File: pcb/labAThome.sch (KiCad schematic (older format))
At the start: 107 parts, among them J1 I2C, J11 24.5.GND.3, J12 NEOPIXEL, J13 Power Input 1, J14 Conn_Coaxial, J15 WS2812_OUT, J2 SRVx, J3 5V, J4 EXT, J5 VPS, J6 FAN2, J7 1wire, J8 1wire, J9 FAN1, K1 G5V-2, K2 G5V-2, K3 G5V-2, M3 SN65HVD230_MODULE, Q1 BC847, Q2 IRLZ44N, Q3 IRLML6344, Q4 BC847, Q5 IRF530, Q6 IRLML5203, SW1 RED, SW2 GREEN, SW4 BLUE, SW5 WHITE, SW7 ROTENC, U1 SR602, U10 MAX3485_MODULE, U11 AM312, U12 24V->4V, U13 LM358, U14 MS4525DO, U15 CCS811_MODULE, U16 24V->5V, U17 DS18B20, U2 TPS5430DDA, U3 Power Input 2, U4 ESP32_DEVKITC_COMPATIBLE, U6 GY-302, U7 Display, U8 MIC, U9 RFM95W-868S2, X1 FAN_6024, m1 Attribution

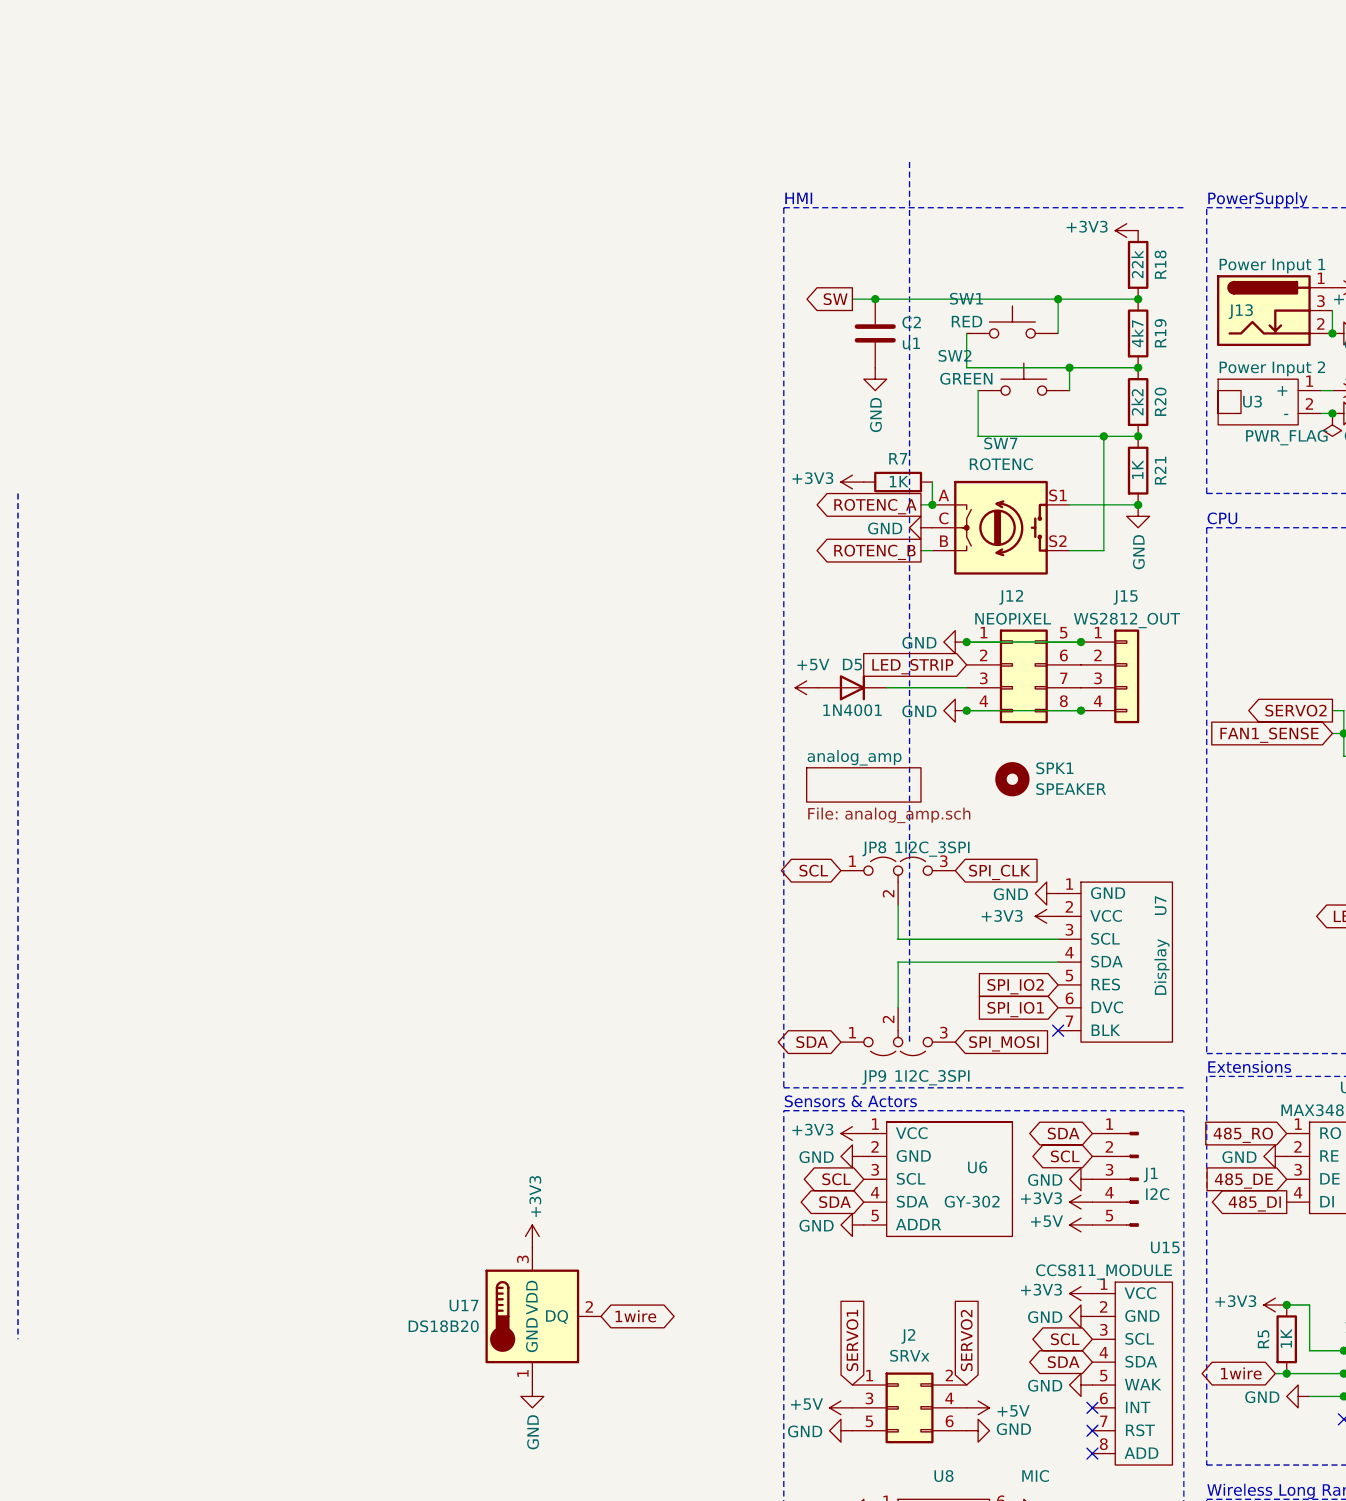
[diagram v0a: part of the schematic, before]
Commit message: Minor PCB update
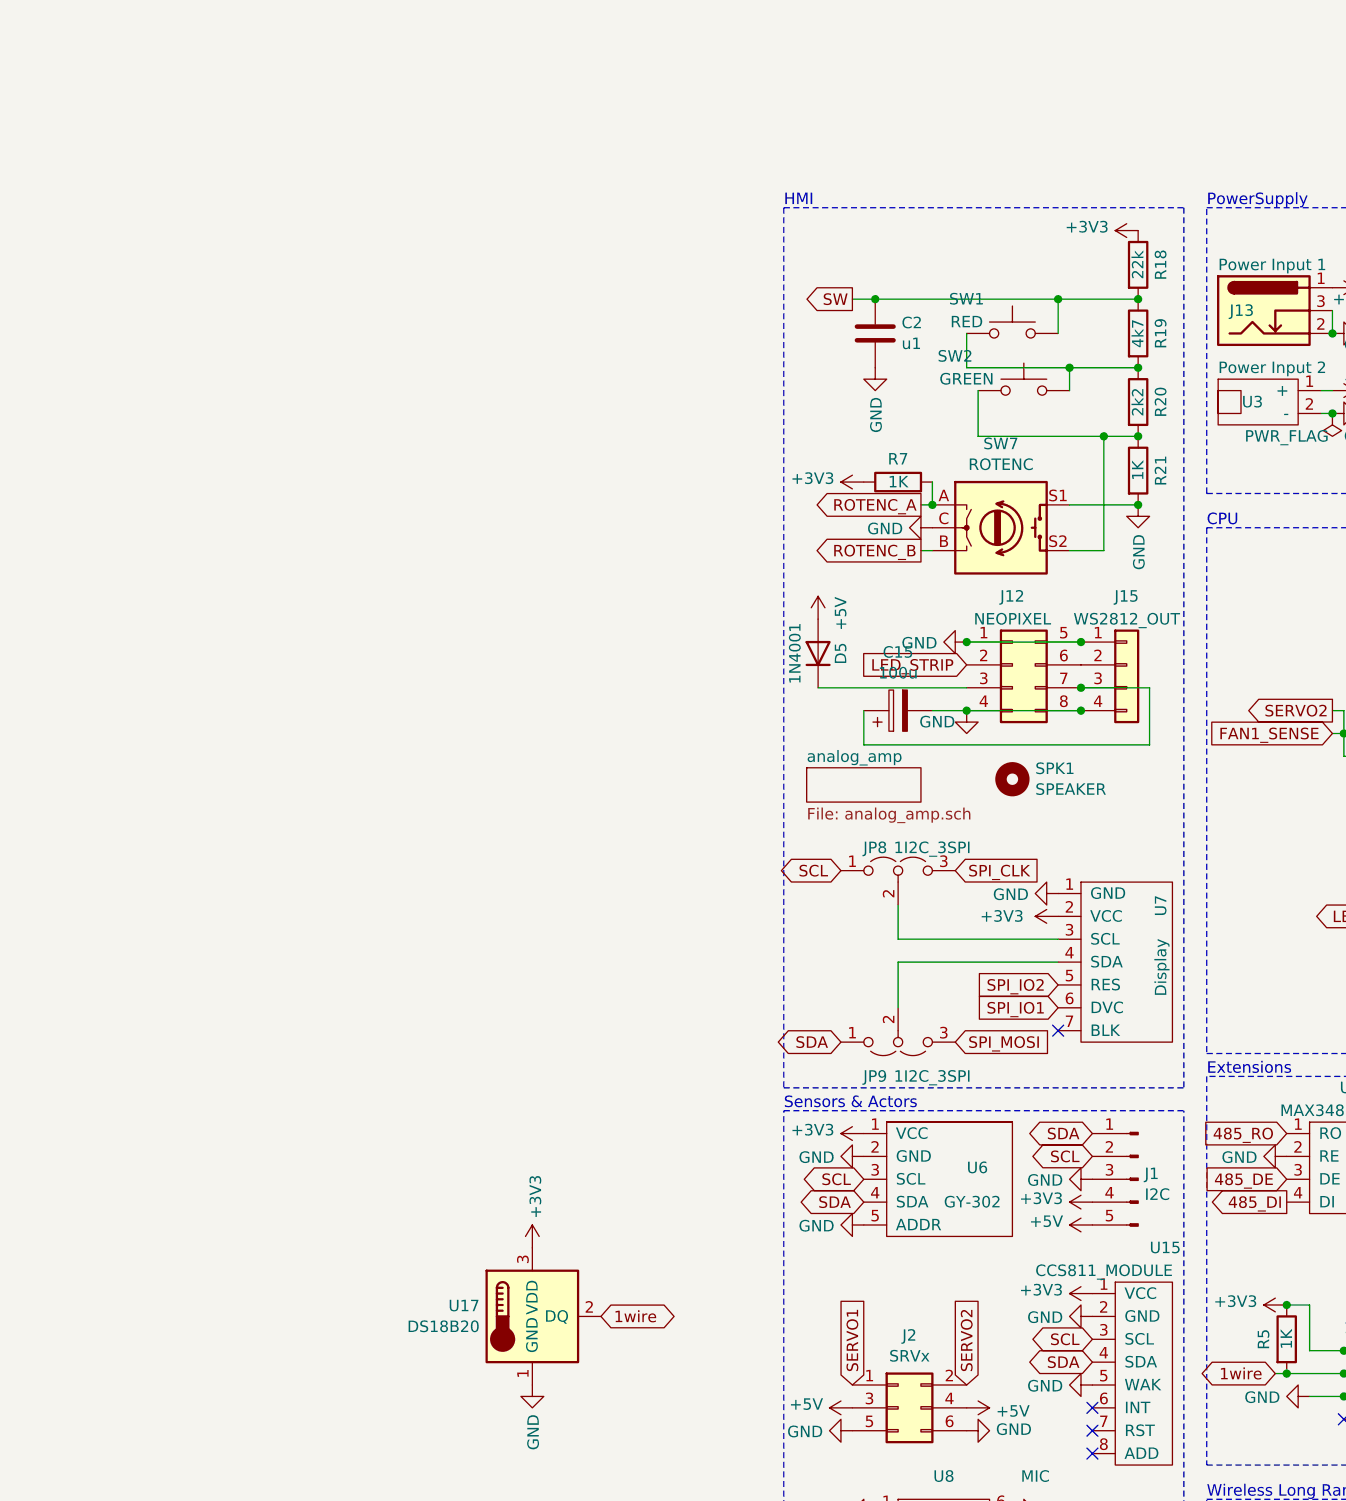
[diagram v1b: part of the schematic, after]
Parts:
- added C15: 100u, liebler_PASSIVES:CP_Elec_6.3x7.7_handsolder, symbol Device:CP
- J12: footprint smopla:NEOPIXEL_STICK_alternativ -> liebler_MODULES:NEOPIXEL_STICK
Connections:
- net GND: now also C15.2
- net at J12.7 (Pin_7), J15.3 (Pin_3): now also C15.1
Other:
- moved on the sheet: D5
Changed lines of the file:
@@
 	1    0    0    -1
 $EndComp
-Wire Notes Line
-	-2800 1850 -2800 5550
 $Comp
 L power:GND #PWR0109
@@
 L power:+5V #PWR051
 U 1 1 5EFC1FD4
-P 700 2700
-F 0 "#PWR051" H 700 2550 50  0001 C CNN
-F 1 "+5V" V 800 2650 50  0000 L CNN
-F 2 "" H 700 2700 50  0001 C CNN
-F 3 "" H 700 2700 50  0001 C CNN
-	1    700  2700
-	0    -1   -1   0
+P 700 2400
+F 0 "#PWR051" H 700 2250 50  0001 C CNN
+F 1 "+5V" V 800 2350 50  0000 L CNN
+F 2 "" H 700 2400 50  0001 C CNN
+F 3 "" H 700 2400 50  0001 C CNN
+	1    700  2400
+	1    0    0    -1
 $EndComp
 $Comp
@@
 P 1350 2800
 F 0 "#PWR052" H 1350 2550 50  0001 C CNN
-F 1 "GND" V 1355 2672 50  0000 R CNN
+F 1 "GND" H 1300 2750 50  0000 R CNN
 F 2 "" H 1350 2800 50  0001 C CNN
 F 3 "" H 1350 2800 50  0001 C CNN
 	1    1350 2800
-	0    1    1    0
+	1    0    0    -1
 $EndComp
 $Comp
@@
 L Diode:1N4001 D5
 U 1 1 5EFF290C
-P 850 2700
-F 0 "D5" H 850 2600 50  0000 C CNN
-F 1 "1N4001" H 850 2800 50  0000 C CNN
-F 2 "Diode_SMD:D_SMA_Handsoldering" H 850 2525 50  0001 C CNN
-F 3 "http://www.vishay.com/docs/88503/1n4001.pdf" H 850 2700 50  0001 C CNN
-	1    850  2700
-	-1   0    0    1
+P 700 2550
+F 0 "D5" H 700 2450 50  0000 C CNN
+F 1 "1N4001" H 700 2650 50  0000 C CNN
+F 2 "Diode_SMD:D_SMA_Handsoldering" H 700 2375 50  0001 C CNN
+F 3 "http://www.vishay.com/docs/88503/1n4001.pdf" H 700 2550 50  0001 C CNN
+	1    700  2550
+	0    -1   -1   0
 $EndComp
 $Comp
@@
 SPI_IO2
 NoConn ~ 1750 4200
-Wire Wire Line
-	1350 2700 1000 2700
 Wire Wire Line
 	7900 3100 7900 3200
@@
 F 0 "J12" H 1550 2900 50  0000 C CNN
 F 1 "NEOPIXEL" H 1550 2800 50  0000 C CNN
-F 2 "smopla:NEOPIXEL_STICK_alternativ" H 1550 2600 50  0001 C CNN
+F 2 "liebler_MODULES:NEOPIXEL_STICK" H 1550 2600 50  0001 C CNN
 F 3 "~" H 1550 2600 50  0001 C CNN
 	1    1550 2600
@@
 $EndComp
 Wire Notes Line
-	1100 400  1100 4250
+	2300 600  2300 4450
 Wire Notes Line
 	550  600  550  4450
@@
 F1 "analog_amp.sch" 50
 $EndSheet
+$Comp
+L Device:CP C15
+U 1 1 60C23DBB
+P 1050 2800
+F 0 "C15" V 1305 2800 50  0000 C CNN
+F 1 "100u" V 1214 2800 50  0000 C CNN
+F 2 "liebler_PASSIVES:CP_Elec_6.3x7.7_handsolder" H 1088 2650 50  0001 C CNN
+F 3 "~" H 1050 2800 50  0001 C CNN
+	1    1050 2800
+	0    -1   -1   0
+$EndComp
+Wire Wire Line
+	1350 2800 1200 2800
+Wire Wire Line
+	700  2700 1350 2700
+Wire Wire Line
+	1850 2700 2150 2700
+Wire Wire Line
+	2150 2700 2150 2950
+Wire Wire Line
+	2150 2950 900  2950
+Wire Wire Line
+	900  2950 900  2800
+Connection ~ 1850 2700
 $EndSCHEMATC

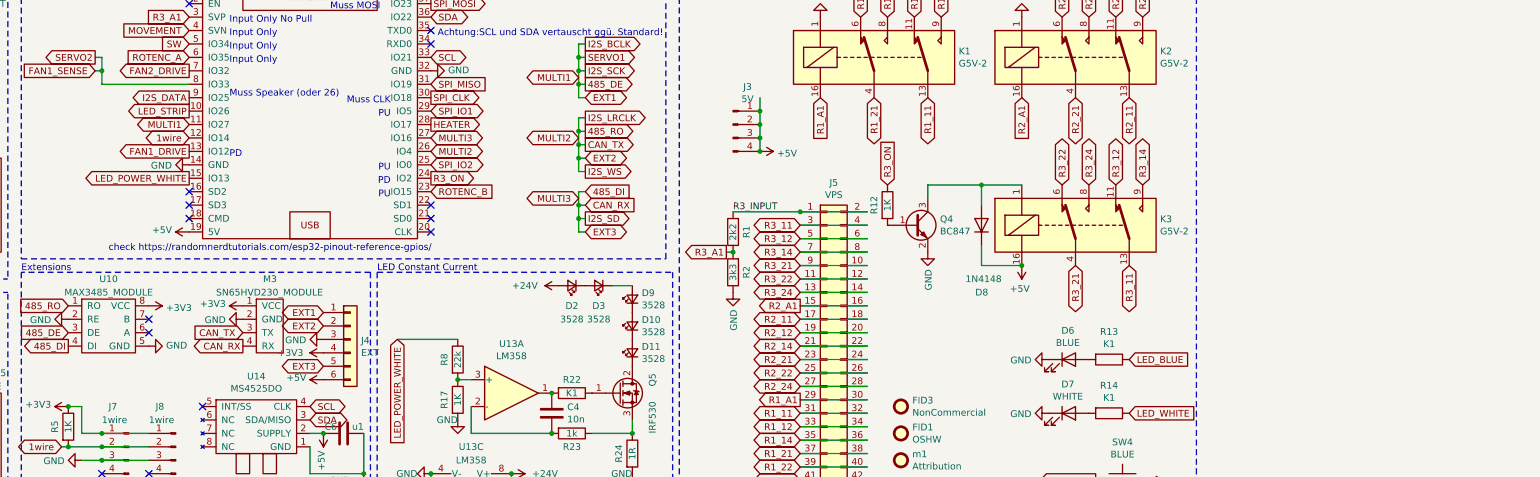
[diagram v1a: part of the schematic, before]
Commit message: labathome V6 as ordered at JLCPCB
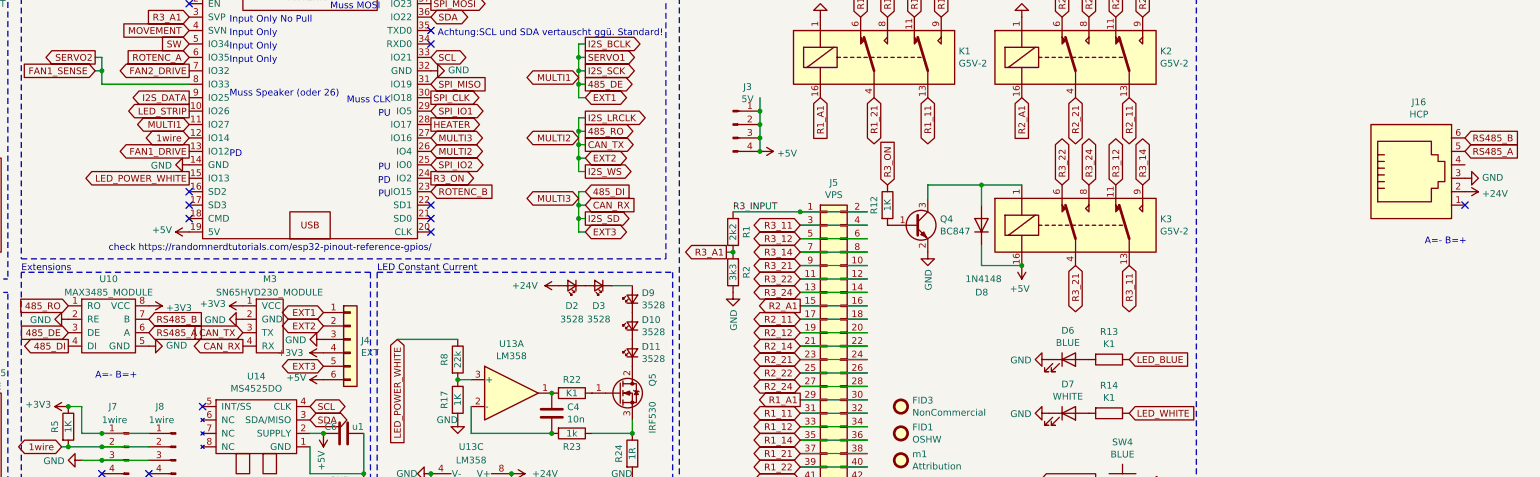
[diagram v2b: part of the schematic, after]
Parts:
- added J16: HCP, liebler_CONN:WR_MJ_Modular_Jack_Vertical_Plastic_6P6C, symbol Connector:6P6C
- SW1, SW2, SW4, SW5: footprint Button_Switch_THT:SW_PUSH-12mm -> liebler_MECH:Button_12mm_ANCHOR_CENTER
- SW7: footprint smopla:RotaryEncoder_Alps_EC11E-Switch_Vertical_H20mm -> liebler_MECH:RotaryEncoder_Alps_EC11E-Switch_Vertical_H20mm
- U1: footprint smopla:SR602 -> liebler_MODULES:PIR_Sensor_SR602
- U4: footprint smopla:ESP32_DEVKITC_COMPATIBLE -> liebler_MODULES:ESP32_DEVKITC_COMPATIBLE
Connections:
- net +24V: now also J16.2
- net GND: now also J16.3
- net RS485_A: now reaches U10.6 (A)
- net RS485_A: now also J16.5
- net RS485_B: now reaches U10.7 (B)
- net RS485_B: now also J16.6
- no-connect marks 33 -> 32
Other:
- note added: "A=- B=+"
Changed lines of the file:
@@
 F 0 "SW1" H 1750 1300 50  0000 C CNN
 F 1 "RED" H 1750 1200 50  0000 C CNN
-F 2 "Button_Switch_THT:SW_PUSH-12mm" H 1550 1350 50  0001 C CNN
+F 2 "liebler_MECH:Button_12mm_ANCHOR_CENTER" H 1550 1350 50  0001 C CNN
 F 3 "~" H 1550 1350 50  0001 C CNN
 	1    1550 1150
@@
 F 0 "SW2" H 1300 1550 50  0000 C CNN
 F 1 "GREEN" H 1350 1450 50  0000 C CNN
-F 2 "Button_Switch_THT:SW_PUSH-12mm" H 1600 1600 50  0001 C CNN
+F 2 "liebler_MECH:Button_12mm_ANCHOR_CENTER" H 1600 1600 50  0001 C CNN
 F 3 "~" H 1600 1600 50  0001 C CNN
 	1    1600 1400
@@
 F 0 "SW5" H 10600 6635 50  0000 C CNN
 F 1 "WHITE" H 10600 6544 50  0000 C CNN
-F 2 "Button_Switch_THT:SW_PUSH-12mm" H 10600 6550 50  0001 C CNN
+F 2 "liebler_MECH:Button_12mm_ANCHOR_CENTER" H 10600 6550 50  0001 C CNN
 F 3 "~" H 10600 6550 50  0001 C CNN
 	1    10600 6350
@@
 F 0 "SW4" H 10600 6235 50  0000 C CNN
 F 1 "BLUE" H 10600 6144 50  0000 C CNN
-F 2 "Button_Switch_THT:SW_PUSH-12mm" H 10600 6150 50  0001 C CNN
+F 2 "liebler_MECH:Button_12mm_ANCHOR_CENTER" H 10600 6150 50  0001 C CNN
 F 3 "~" H 10600 6150 50  0001 C CNN
 	1    10600 5950
@@
 F 0 "U4" H 4550 4325 50  0000 C CNN
 F 1 "ESP32_DEVKITC_COMPATIBLE" H 4550 4234 50  0000 C CNN
-F 2 "smopla:ESP32_DEVKITC_COMPATIBLE" H 4550 3050 50  0001 C CNN
+F 2 "liebler_MODULES:ESP32_DEVKITC_COMPATIBLE" H 4550 3050 50  0001 C CNN
 F 3 "" H 4550 3050 50  0001 C CNN
 	1    4550 3200
@@
 F 0 "U1" H 742 7465 50  0000 C CNN
 F 1 "SR602" H 742 7374 50  0000 C CNN
-F 2 "smopla:SR602" H 800 7100 50  0001 C CNN
+F 2 "liebler_MODULES:PIR_Sensor_SR602" H 800 7100 50  0001 C CNN
 F 3 "" H 800 7100 50  0001 C CNN
 	1    800  7100
@@
 	0    1    1    0
 $EndComp
-NoConn ~ 3350 4850
-NoConn ~ 3350 4750
 $Comp
 L power:GND #PWR0116
@@
 F 0 "SW7" H 1500 2367 50  0000 C CNN
 F 1 "ROTENC" H 1500 2276 50  0000 C CNN
-F 2 "smopla:RotaryEncoder_Alps_EC11E-Switch_Vertical_H20mm" H 1350 2160 50  0001 C CNN
+F 2 "liebler_MECH:RotaryEncoder_Alps_EC11E-Switch_Vertical_H20mm" H 1350 2160 50  0001 C CNN
 F 3 "~" H 1500 2260 50  0001 C CNN
 	1    1500 2000
@@
 	900  2950 900  2800
 Connection ~ 1850 2700
+$Comp
+L Connector:6P6C J16
+U 1 1 610E3B2A
+P 12750 3700
+F 0 "J16" H 12807 4267 50  0000 C CNN
+F 1 "HCP" H 12807 4176 50  0000 C CNN
+F 2 "liebler_CONN:WR_MJ_Modular_Jack_Vertical_Plastic_6P6C" V 12750 3725 50  0001 C CNN
+F 3 "~" V 12750 3725 50  0001 C CNN
+	1    12750 3700
+	1    0    0    -1
+$EndComp
+Text Notes 2950 5200 0    50   ~ 0
+A=- B=+
+NoConn ~ 13150 3900
+$Comp
+L power:+24V #PWR0106
+U 1 1 6110EDB7
+P 13150 3800
+F 0 "#PWR0106" H 13150 3650 50  0001 C CNN
+F 1 "+24V" V 13165 3928 50  0000 L CNN
+F 2 "" H 13150 3800 50  0001 C CNN
+F 3 "" H 13150 3800 50  0001 C CNN
+	1    13150 3800
+	0    1    1    0
+$EndComp
+$Comp
+L power:GND #PWR0107
+U 1 1 6110F531
+P 13150 3700
+F 0 "#PWR0107" H 13150 3450 50  0001 C CNN
+F 1 "GND" V 13155 3572 50  0000 R CNN
+F 2 "" H 13150 3700 50  0001 C CNN
+F 3 "" H 13150 3700 50  0001 C CNN
+	1    13150 3700
+	0    -1   -1   0
+$EndComp
+Text GLabel 13150 3500 2    50   Input ~ 0
+RS485_A
+Text GLabel 13150 3400 2    50   Input ~ 0
+RS485_B
+Text Notes 12850 4200 0    50   ~ 0
+A=- B=+
+Text GLabel 3350 4850 2    50   Input ~ 0
+RS485_A
+Text GLabel 3350 4750 2    50   Input ~ 0
+RS485_B
 $EndSCHEMATC
